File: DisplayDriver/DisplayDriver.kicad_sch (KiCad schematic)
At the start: 46 parts, among them J1 HTSS-108-01-G-D, J2 HEADER-1X14, J3 HTSS-108-01-G-D, J4 Molex, U1 ESP32-S3-WROOM-1, U2 74AHCT245, U3 74AHCT245, U4 AMS1117-3.3, U5 AP2112K-3.3, X2 UJ20-C-H-G-SMT-TR

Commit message: I swear this is the last PCB revision
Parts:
- added C999b1: C, Capacitor_SMD:C_0805_2012Metric_Pad1.18x1.45mm_HandSolder, symbol DisplayLibrary(sketch):CAP_CERAMIC0603_NO
- added C999d1: C, Capacitor_SMD:C_0603_1608Metric, symbol DisplayLibrary(sketch):C_Small
- added MOL3: CASE_SW, Connector_Molex:Molex_KK-254_AE-6410-02A_1x02_P2.54mm_Vertical, symbol DisplayLibrary(sketch):SW_Push
- 5Vin1: symbol Connector:Barrel_Jack -> DisplayLibrary(sketch):Barrel_Jack
- BOOT1, RST1: value (Generic) Lab Kit -> Lab Kit
- C12: renamed from C4; symbol Device:C -> DisplayLibrary(sketch):C
- C12B1: renamed from C3; symbol Device:C -> DisplayLibrary(sketch):C
- C13: renamed from C11; symbol Device:C -> DisplayLibrary(sketch):C
- C13B1: renamed from C5; symbol Device:C -> DisplayLibrary(sketch):C
- MOL1: renamed from UP1; value SW_Push -> CASE_SW
- MOL2: renamed from DOWN1; value SW_Push -> CASE_SW
- MOL4: renamed from J4; value Molex -> Vin; symbol Connector:Conn_01x02_Pin -> DisplayLibrary(sketch):Conn_01x02_Pin
- U4: symbol Regulator_Linear:AMS1117-3.3 -> DisplayLibrary(sketch):AMS1117-3.3
- U5: symbol Regulator_Linear:AP2112K-3.3 -> DisplayLibrary(sketch):AP2112K-3.3
- renumbered C8 to C1, C9 to C10, C10 to C11, C7 to C2, C17 to C3, C14 to C4, C2 to C5, C1 to C6, C6 to C7, C13 to C8, C16 to C9, PC2 to PC1, R26 to R10, R25 to R11, R28 to R8, R29 to R9
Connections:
- net 3.3V: no longer C13B1.1, U5.5 (VOUT)
- net ADDRA_3V: now also U1.23 (IO21), U2.4 (A3); no longer U1.19 (IO11), U2.3 (A2)
- net ADDRB_3V: now also U1.24 (IO47), U2.3 (A2); no longer U1.18 (IO10), U2.4 (A3)
- net ADDRC_3V: now also U1.21 (IO13), U2.6 (A5); no longer U1.17 (IO9), U2.5 (A4)
- net ADDRD_3V: now also U1.22 (IO14), U2.5 (A4); no longer U1.5 (IO5), U2.6 (A5)
- net B2_3V: now also U1.25 (IO48); no longer U1.20 (IO12)
- net CLK: now also U2.12 (B7); no longer U2.13 (B6)
- net CLK_3V: now also U1.19 (IO11), U2.8 (A7); no longer U1.12 (IO8), U2.7 (A6)
- net G1_3V: now also U1.35 (IO42), U3.5 (A4); no longer U1.32 (IO39), U3.8 (A7)
- net G2_3V: now also U1.32 (IO39), U3.8 (A7); no longer U1.35 (IO42), U3.5 (A4)
- net GND: now also MOL3.1
- net LAT: now also U2.13 (B6); no longer U2.12 (B7)
- net LAT_3V: now also U1.20 (IO12), U2.7 (A6); no longer U1.11 (IO18), U2.8 (A7)
- net M1_A: now also U2.16 (B3); no longer U2.17 (B2)
- net M1_B: now also U2.17 (B2); no longer U2.16 (B3)
- net M1_C: now also U2.14 (B5); no longer U2.15 (B4)
- net M1_D: now also U2.15 (B4); no longer U2.14 (B5)
- net M1_G1: now also U3.15 (B4); no longer U3.12 (B7)
- net M1_G2: now also U3.12 (B7); no longer U3.15 (B4)
- net M1_R1: now also U3.14 (B5); no longer U3.11 (B8)
- net M1_R2: now also U3.11 (B8); no longer U3.14 (B5)
- net OE_3V: now also U1.18 (IO10); no longer U1.10 (IO17)
- net R1_3V: now also U1.34 (IO41), U3.6 (A5); no longer U1.31 (IO38), U3.9 (A8)
- net R2_3V: now also U1.31 (IO38), U3.9 (A8); no longer U1.34 (IO41), U3.6 (A5)
- net D13 renamed D9
- net D9: now also U1.17 (IO9); no longer U1.21 (IO13)
- net DOWN renamed A1
- net UP renamed A0
- new net: C13B1.1, U5.5 (VOUT)
- new net A2: MOL3.2, U1.10 (IO17)
- no-connect marks 25 -> 30
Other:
- note added: "3.3V REGULATOR"
- note added: "5V IN"
- note added: "BATTERY"
- note added: "Caps for screen power??"
- note added: "IDC OUTPUT"
- note added: "POWER & D09 LEDS"
- note added: "TACT SWITCHES (molex to case)"
- note added: "bulk"
- note added: "dcpl"
- note added: "neopxl LED (boot status)"
- note added: "ref:"
- note added: "spare IDC for debug"
- note removed: "Caps for screen power"
- note removed: "IDC OUTPUT (HUB75)"
- note removed: "POWER & D13 LEDS"
- note removed: "TACT SWITCHES"
- note removed: "TO DO: (this is all board exluded!)"
- note removed: "neopxl LED (bootloader)"
- note removed: "spare for debug (if space on board)"
- note removed: "this needs to be done properly:"
- moved on the sheet: 5Vin1, BOOT1, BT1, C1, C10, C11, C12, C12B1, C13, C13B1, C2, C4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

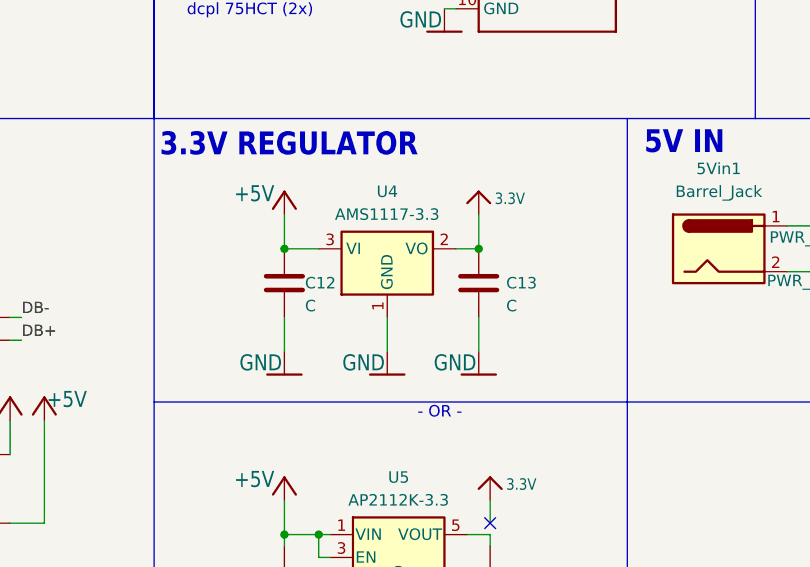
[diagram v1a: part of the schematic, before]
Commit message: e
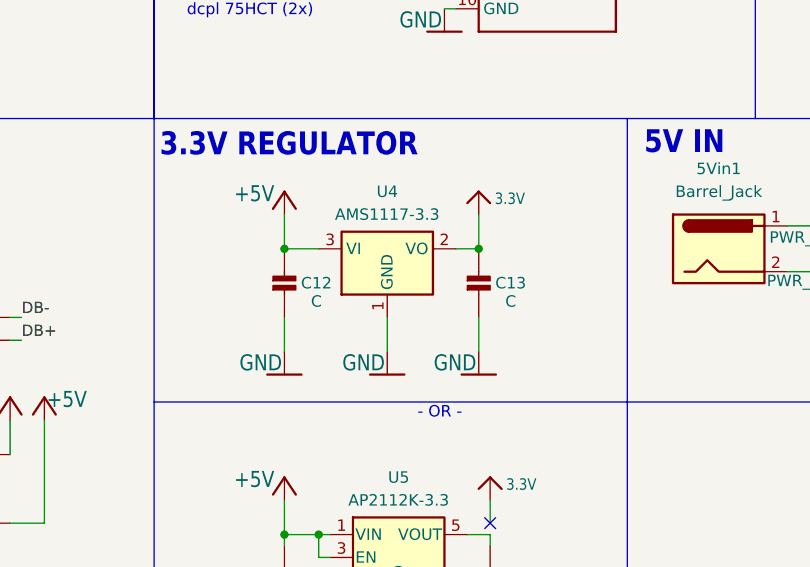
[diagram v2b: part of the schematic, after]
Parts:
- removed C12, C13: C, Capacitor_SMD:C_0805_2012Metric_Pad1.18x1.45mm_HandSolder, symbol DisplayLibrary(sketch):C
- added C12, C13: C, Capacitor_SMD:C_0805_2012Metric_Pad1.18x1.45mm_HandSolder, symbol DisplayLibrary(sketch):CAP_CERAMIC0603_NO
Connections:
- net +5V: now also C12.1
- net 3.3V: now also C13.1
- net GND: now also C12.2, C13.2
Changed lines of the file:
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@@
 	)
 	(junction
-		(at 86.36 129.54)
-		(diameter 0)
-		(color 0 0 0 0)
-	)
-	(junction
-		(at 107.95 129.54)
-		(diameter 0)
-		(color 0 0 0 0)
-	)
-	(junction
 		(at 86.36 161.29)
 		(diameter 0)
@@
 	)
 	(junction
+		(at 86.36 129.54)
+		(diameter 0)
+		(color 0 0 0 0)
+	)
+	(junction
 		(at 105.41 82.55)
 		(diameter 0)
 		(color 0 0 0 0)
 	)
+	(junction
+		(at 107.95 129.54)
+		(diameter 0)
+		(color 0 0 0 0)
+	)
 	(no_connect
 		(at 274.32 83.82)
@@
 	)
 	(symbol
+		(lib_id "DisplayLibrary(sketch):CAP_CERAMIC0603_NO")
+		(at 86.36 134.62 0)
+		(unit 1)
+		(exclude_from_sim no)
+		(in_bom yes)
+		(on_board yes)
+		(dnp no)
+		(property "Reference" "C12"
+			(at 89.916 133.35 0)
+			(effects
+				(font
+					(size 1.27 1.27)
+				)
+			)
+		)
+		(property "Value" "C"
+			(at 89.916 135.382 0)
+			(effects
+				(font
+					(size 1.27 1.27)
+				)
+			)
+		)
+		(property "Footprint" "Capacitor_SMD:C_0805_2012Metric_Pad1.18x1.45mm_HandSolder"
+			(at 86.36 134.62 0)
+			(effects
+				(font
+					(size 1.27 1.27)
+				)
+				(hide yes)
+			)
+		)
+		(property "Datasheet" ""
+			(at 86.36 134.62 0)
+			(effects
+				(font
+					(size 1.27 1.27)
+				)
+				(hide yes)
+			)
+		)
+		(property "Description" ""
+			(at 86.36 134.62 0)
+			(effects
+				(font
+					(size 1.27 1.27)
+				)
+				(hide yes)
+			)
+		)
+		(pin "1"
+		)
+		(pin "2"
+		)
+		(instances
+			(project "DisplayDriver"
+				(path "/ddc4c194-bb30-4734-adb1-ce29ad370a60"
+					(reference "C12")
+					(unit 1)
+				)
+			)
+		)
+	)
+	(symbol
 		(lib_id "DisplayLibrary(sketch):CAP_CERAMIC0805-NOOUTLINE")
 		(at 77.47 63.5 180)
@@
 	(symbol
 		(lib_id "DisplayLibrary(sketch):C")
-		(at 86.36 133.35 0)
-		(unit 1)
-		(exclude_from_sim no)
-		(in_bom yes)
-		(on_board yes)
-		(dnp no)
-		(property "Reference" "C12"
-			(at 88.646 133.35 0)
-			(effects
-				(font
-					(size 1.27 1.27)
-				)
-				(justify left)
-			)
-		)
-		(property "Value" "C"
-			(at 88.646 135.89 0)
-			(effects
-				(font
-					(size 1.27 1.27)
-				)
-				(justify left)
-			)
-		)
-		(property "Footprint" "Capacitor_SMD:C_0805_2012Metric_Pad1.18x1.45mm_HandSolder"
-			(at 87.3252 137.16 0)
-			(effects
-				(font
-					(size 1.27 1.27)
-				)
-				(hide yes)
-			)
-		)
-		(property "Datasheet" "~"
-			(at 86.36 133.35 0)
-			(effects
-				(font
-					(size 1.27 1.27)
-				)
-				(hide yes)
-			)
-		)
-		(property "Description" "Unpolarized capacitor"
-			(at 86.36 133.35 0)
-			(effects
-				(font
-					(size 1.27 1.27)
-				)
-				(hide yes)
-			)
-		)
-		(pin "2"
-		)
-		(pin "1"
-		)
-		(instances
-			(project "DisplayDriver"
-				(path "/ddc4c194-bb30-4734-adb1-ce29ad370a60"
-					(reference "C12")
-					(unit 1)
-				)
-			)
-		)
-	)
-	(symbol
-		(lib_id "DisplayLibrary(sketch):C")
 		(at 86.36 166.37 0)
 		(unit 1)
@@
 	)
 	(symbol
-		(lib_id "DisplayLibrary(sketch):C")
-		(at 107.95 133.35 0)
-		(unit 1)
-		(exclude_from_sim no)
-		(in_bom yes)
-		(on_board yes)
-		(dnp no)
-		(property "Reference" "C13"
-			(at 110.998 133.35 0)
-			(effects
-				(font
-					(size 1.27 1.27)
-				)
-				(justify left)
-			)
-		)
-		(property "Value" "C"
-			(at 110.998 135.89 0)
-			(effects
-				(font
-					(size 1.27 1.27)
-				)
-				(justify left)
-			)
-		)
-		(property "Footprint" "Capacitor_SMD:C_0805_2012Metric_Pad1.18x1.45mm_HandSolder"
-			(at 108.9152 137.16 0)
-			(effects
-				(font
-					(size 1.27 1.27)
-				)
-				(hide yes)
-			)
-		)
-		(property "Datasheet" "~"
-			(at 107.95 133.35 0)
-			(effects
-				(font
-					(size 1.27 1.27)
-				)
-				(hide yes)
-			)
-		)
-		(property "Description" "Unpolarized capacitor"
-			(at 107.95 133.35 0)
-			(effects
-				(font
-					(size 1.27 1.27)
-				)
-				(hide yes)
-			)
-		)
-		(pin "2"
-		)
-		(pin "1"
-		)
-		(instances
-			(project "DisplayDriver"
-				(path "/ddc4c194-bb30-4734-adb1-ce29ad370a60"
-					(reference "C13")
-					(unit 1)
-				)
-			)
-		)
-	)
-	(symbol
 		(lib_id "DisplayLibrary(sketch):PowerTags_+5V")
 		(at 77.47 31.75 0)
@@
 					(unit 1)
 				)
+			)
+		)
+	)
+	(symbol
+		(lib_id "DisplayLibrary(sketch):CAP_CERAMIC0603_NO")
+		(at 107.95 134.62 0)
+		(unit 1)
+		(exclude_from_sim no)
+		(in_bom yes)
+		(on_board yes)
+		(dnp no)
+		(property "Reference" "C13"
+			(at 111.506 133.35 0)
+			(effects
+				(font
+					(size 1.27 1.27)
+				)
+			)
+		)
+		(property "Value" "C"
+			(at 111.506 135.382 0)
+			(effects
+				(font
+					(size 1.27 1.27)
+				)
+			)
+		)
+		(property "Footprint" "Capacitor_SMD:C_0805_2012Metric_Pad1.18x1.45mm_HandSolder"
+			(at 107.95 134.62 0)
+			(effects
+				(font
+					(size 1.27 1.27)
+				)
+				(hide yes)
+			)
+		)
+		(property "Datasheet" ""
+			(at 107.95 134.62 0)
+			(effects
+				(font
+					(size 1.27 1.27)
+				)
+				(hide yes)
+			)
+		)
+		(property "Description" ""
+			(at 107.95 134.62 0)
+			(effects
+				(font
+					(size 1.27 1.27)
+				)
+				(hide yes)
+			)
+		)
+		(pin "1"
+		)
+		(pin "2"
+		)
+		(instances
+			(project "DisplayDriver"
+				(path "/ddc4c194-bb30-4734-adb1-ce29ad370a60"
+					(reference "C13")
+					(unit 1)
+				)
